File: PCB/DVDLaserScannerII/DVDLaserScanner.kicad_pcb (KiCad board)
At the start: 2 copper layers, 144 x 80 mm, 83 parts, among them Q1 Q_NMOS_GDS, SW1 BUT, U1 MCP4922-E/SL, U10 Con45, U11 Con45, U13 TLC2274, U2 MCP4922-E/SL, U3 ARDUINO_MICRO, U4 TCA0372_DWG, U5 TCA0372_DWG, U6 TCA0372_DWG, U7 MCP6002, U8 MCP4922-E/SL, U9 TLC2274, X1 MountPad3, X2 MountPad3, X3 MountPad3, X4 MountPad3, X5 PAD, X6 PAD, X7 PAD

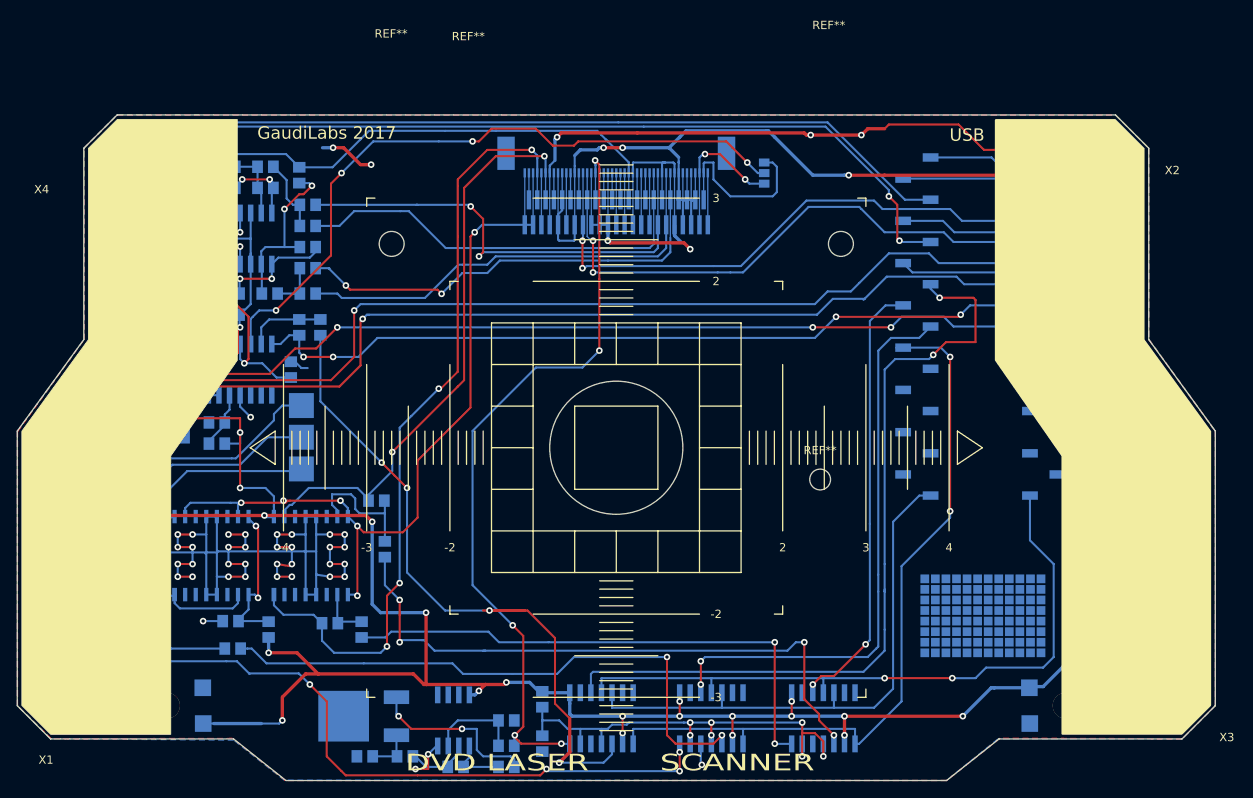
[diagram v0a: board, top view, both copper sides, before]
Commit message: Update schematic
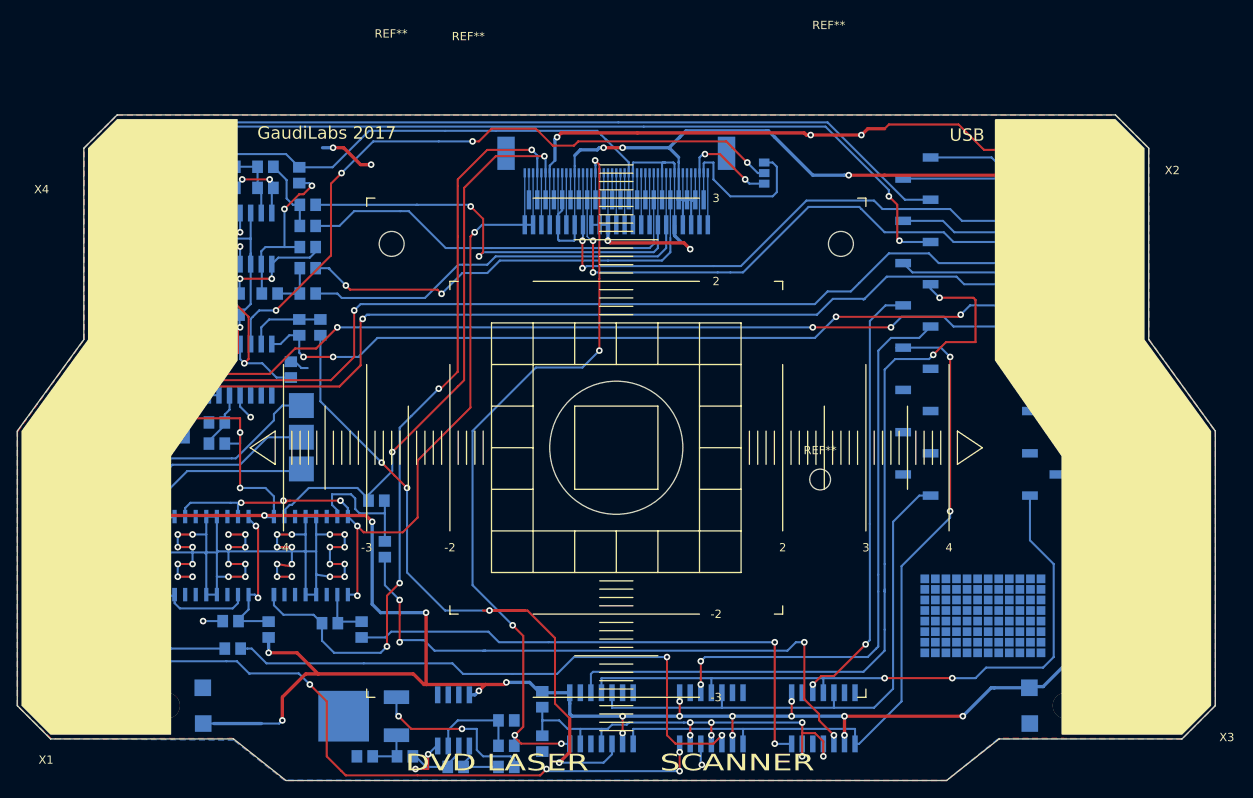
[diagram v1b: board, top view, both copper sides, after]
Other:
- net class Default removed
- net class PWR removed
- net class Thin removed
